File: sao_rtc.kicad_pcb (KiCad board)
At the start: 2 copper layers, 44.9 x 32.9 mm, 40 parts, among them J1 S2B-PH-K-S(LF)(SN), J2 Conn_02x03_Odd_Even, J3 Conn_02x03_Odd_Even, P1 USB_C_Plug_USB2.0, SW1 DPDT, U1 AW32001ECSR, U2 PCF8563DRG, U3 M3410, Y1 32.768 kHz

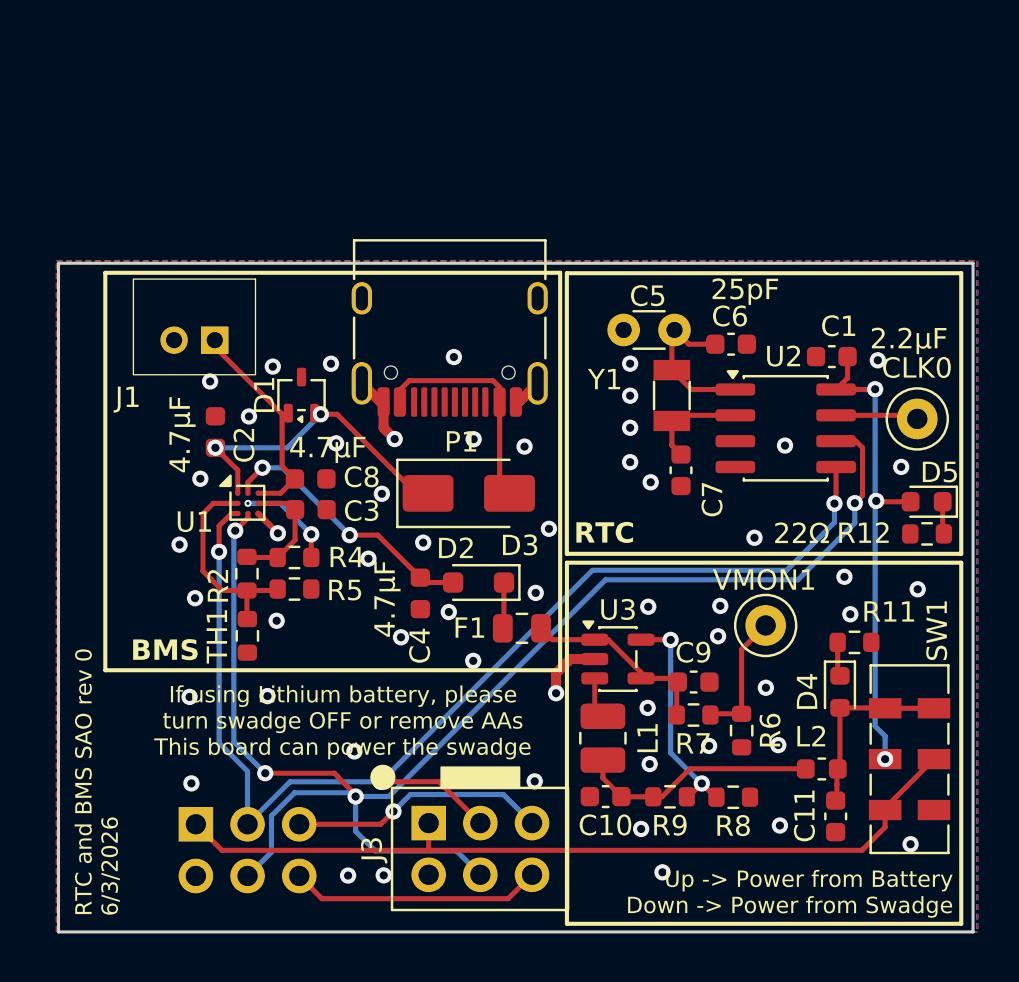
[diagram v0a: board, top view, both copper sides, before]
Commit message: Complete 1st Draft
First Draft at Schematic Capture and Layout
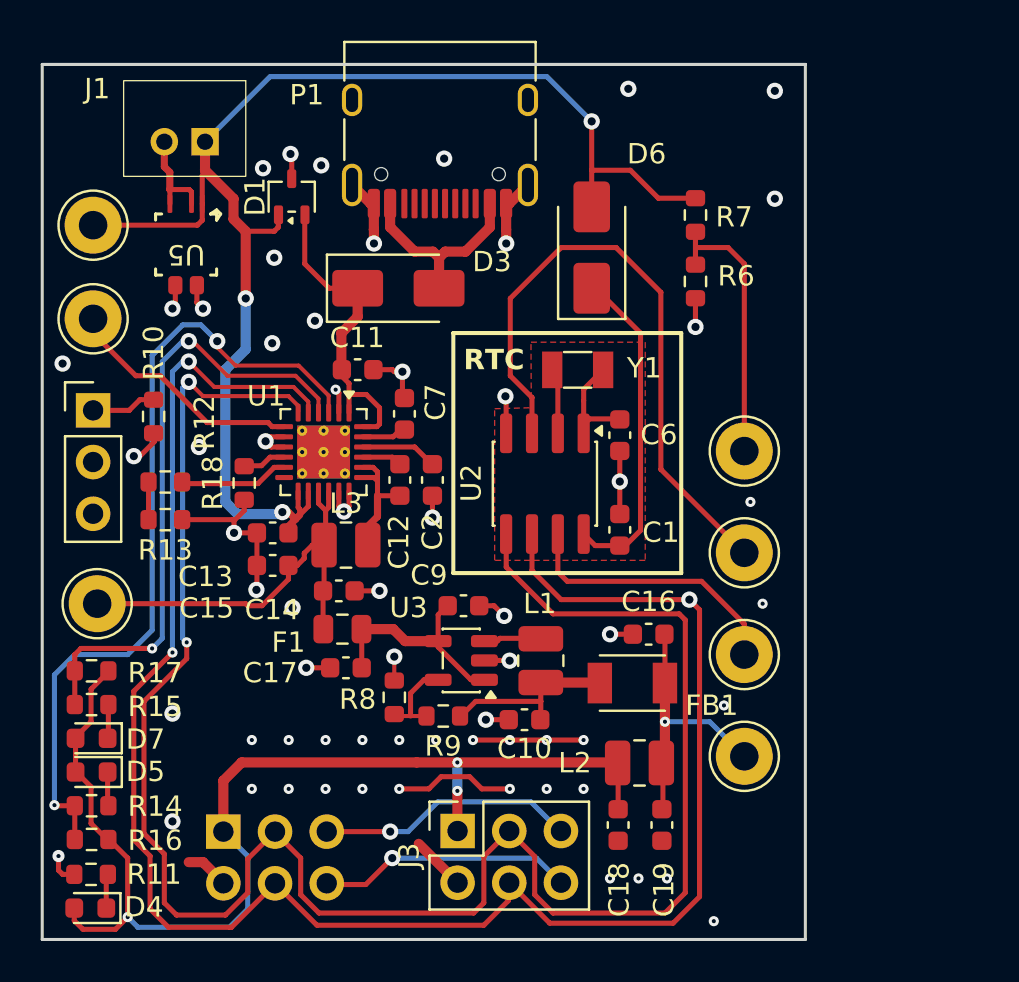
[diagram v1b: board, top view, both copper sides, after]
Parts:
- removed C3: 1μF, sao:C_0603_1608Metric
- removed C4, C8: 4.7μF, sao:C_0603_1608Metric
- removed C5: C, Capacitor_THT:C_Disc_D3.0mm_W1.6mm_P2.50mm
- removed CLK0, VMON1: TestPoint, TestPoint:TestPoint_Loop_D2.50mm_Drill1.0mm
- removed D2: 4.3V, Diode_SMD:D_SOD-323_HandSoldering
- removed R2, R5: Ω, Resistor_SMD:R_0603_1608Metric
- removed R4: 10kΩ, Resistor_SMD:R_0603_1608Metric
- removed SW1: DPDT, Button_Switch_SMD:SW_DPDT_CK_JS202011JCQN
- removed TH1: Thermistor_NTC, Resistor_SMD:R_0603_1608Metric
- added C12: 47nF, Capacitor_SMD:C_0603_1608Metric, F.Cu at (97.6, 71.4)
- added C13: 10uF, Capacitor_SMD:C_0603_1608Metric, F.Cu at (91.3, 74.0)
- added C14: 10uF, Capacitor_SMD:C_0603_1608Metric, F.Cu at (94.6, 76.9)
- added C15: 10uF, Capacitor_SMD:C_0603_1608Metric, F.Cu at (91.3, 75.6)
- added C16: 22uF, Capacitor_SMD:C_0603_1608Metric, F.Cu at (109.8, 79.0)
- added C17: 22uF, Capacitor_SMD:C_0603_1608Metric, F.Cu at (94.9, 80.7)
- added C18: 47nF, Capacitor_SMD:C_0603_1608Metric, F.Cu at (108.3, 88.4)
- added C19: 47nF, Capacitor_SMD:C_0603_1608Metric, F.Cu at (110.5, 88.4)
- added D6: D, Diode_SMD:D_SMA, F.Cu at (107.0, 60.0)
- added D7: STAT, LED_SMD:LED_0603_1608Metric, F.Cu at (82.4, 84.1)
- added FB1: FerriteBead, Inductor_SMD:L_TDK_NLV32_3.2x2.5mm, F.Cu at (109.0, 81.4)
- added JP1: PH2.54-1x3P, Connector_PinHeader_2.54mm:PinHeader_1x03_P2.54mm_Vertical, F.Cu at (82.5, 68.0)
- added L3: 1uH, Inductor_SMD:L_1008_2520Metric, F.Cu at (94.9, 74.6)
- added R10: 10kΩ, Resistor_SMD:R_0603_1608Metric, F.Cu at (85.5, 68.3)
- added R12: 5.36k, Resistor_SMD:R_0603_1608Metric, F.Cu at (86.0, 71.5)
- added R13: 31.6k, Resistor_SMD:R_0603_1608Metric, F.Cu at (86.0, 73.4)
- added R15: 22Ω, Resistor_SMD:R_0603_1608Metric, F.Cu at (82.4, 82.5)
- added R16: 10kΩ, Resistor_SMD:R_0603_1608Metric, F.Cu at (82.4, 89.1)
- added R17: 10kΩ, Resistor_SMD:R_0603_1608Metric, F.Cu at (82.4, 80.8)
- added R18: 232, Resistor_SMD:R_0603_1608Metric, F.Cu at (89.9, 71.6)
- added TP1: TestPoint, TestPoint:TestPoint_Loop_D2.60mm_Drill1.4mm_Beaded, F.Cu at (114.5, 80.0)
- added TP2: TestPoint, TestPoint:TestPoint_Loop_D2.60mm_Drill1.4mm_Beaded, F.Cu at (114.5, 75.0)
- added TP3: TP_BATT, TestPoint:TestPoint_Loop_D2.60mm_Drill1.4mm_Beaded, F.Cu at (82.5, 58.9)
- added TP4: TP_PGOOD, TestPoint:TestPoint_Loop_D2.60mm_Drill1.4mm_Beaded, F.Cu at (82.5, 63.5)
- added TP5: TP_BMS, TestPoint:TestPoint_Loop_D2.60mm_Drill1.4mm_Beaded, F.Cu at (82.7, 77.5)
- added TP6: TP_VMON, TestPoint:TestPoint_Loop_D2.60mm_Drill1.4mm_Beaded, F.Cu at (114.5, 70.0)
- added TP7: TP_3V3, TestPoint:TestPoint_Loop_D2.60mm_Drill1.4mm_Beaded, F.Cu at (114.5, 85.0)
- added U5: XB7608AJ, sao:CPC-5_2.6mmx4mm_P0.53mm, F.Cu at (87.1, 59.9)
- C1: value 2.2μF -> 22uF
- C11: value 12uF -> 1μF
- C2: footprint sao:C_0603_1608Metric -> Capacitor_SMD:C_0603_1608Metric
- C7: value ~ -> 10μF
- D5: value RTC ON -> PGOOD
- J2: value Conn_02x03_Odd_Even -> Connector, In
- J3: value Conn_02x03_Odd_Even -> Connector, Out; footprint Swadge_Parts:PinSocket_2x03_P2.54mm_Vertical -> sao:PinHeader_2x03_P2.54mm_Vertical_Flipped
- L2: footprint Inductor_SMD:L_0603_1608Metric -> Inductor_SMD:L_1008_2520Metric
- U1: value AW32001ECSR -> BQ24259; footprint Package_CSP:WLCSP-9_1.21x1.22mm_Layout3x3_P0.4mm -> Package_DFN_QFN:HVQFN-24-1EP_4x4mm_P0.5mm_EP2.6x2.6mm_ThermalVias
- U3: value M3410 -> MT3410
- moved R14 43.2 mm to (82.4, 87.4)
- moved D5 43.1 mm to (82.4, 85.8)
- moved R11 39.2 mm to (82.4, 90.8), turned to 0 degrees
- moved D4 38.3 mm to (82.4, 92.5), turned to 180 degrees
- moved C11 32.1 mm to (95.5, 66.0), turned to 0 degrees
- moved R7 24.6 mm to (112.1, 58.4), turned to 90 degrees
- moved R6 22.2 mm to (112.1, 61.7)
- moved R8 17.4 mm to (97.3, 82.1), turned to -90 degrees
- moved C7 13.9 mm to (97.8, 68.2), turned to 90 degrees
- moved C1 13.5 mm to (108.4, 73.9), turned to 90 degrees
- moved U2 12.1 mm to (104.7, 71.6), turned to -90 degrees
- moved C9 11.9 mm to (100.7, 77.6)
- moved R9 11.8 mm to (99.7, 83.0), turned to 0 degrees
- moved C2 10.9 mm to (99.2, 71.4), turned to -90 degrees
- moved D3 10.7 mm to (97.5, 62.0)
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- renumbered R12 to R14
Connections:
- net Net-(U2-OSCI) renamed /RTC/OSCI
- net Net-(U3-FB) renamed /3V3_REG/FB
- C1 pad 1: VDD -> /RTC/V_RTC
- C10 pad 1: Net-(C10-Pad1) -> /3V3_REG/3V3_SW
- C11 pad 1: 3V3 SAO -> +5V
- C2 pad 1: +5V -> /BMS/REGN
- C7 pad 1: Net-(U2-OSCO) -> /BMS/PMID
- C9 pad 1: SNODE -> /VBMS
- D1 pad 1: BATT+ -> /BATT+
- D4 pad 2: 3V3 SAO -> 3V3
- D5 pad 2: VDD -> 3V3
- F1 pad 1: SNODE -> /BMS/VSYS
- F1 pad 2: Net-(D2-K) -> /VBMS
- J1 pad 1: BATT+ -> /BATT+
- J1 pad 2: GND -> Net-(J1-Pad2)
- J2 pad 3: SDA -> /SDA
- J2 pad 4: SCL -> /SCL
- J3 pad 3: SDA -> /SDA
- J3 pad 4: SCL -> /SCL
- L1 pad 1: Net-(C10-Pad1) -> /3V3_REG/3V3_SW
- L2 pad 1: 3V3 SAO -> 3V3
- L2 pad 2: Net-(C10-Pad1) -> /3V3_SAO
- R14 pad 1: GND -> /~{PG}
- R7 pad 2: SNODE -> /BATT+
- R9 pad 2: Net-(C10-Pad1) -> /3V3_REG/3V3_SW
- U2 pad 2: Net-(U2-OSCO) -> /RTC/OSCO
- U2 pad 3: unconnected-(U2-~{INT}-Pad3) -> /RTC/~{INT}
- U2 pad 5: SDA -> /SDA
- U2 pad 6: SCL -> /SCL
- U2 pad 7: Net-(U2-CLKO) -> /RTC/CLK0
- U2 pad 8: VDD -> /RTC/V_RTC
- U3 pad 1: SNODE -> /VBMS
- U3 pad 4: SNODE -> /VBMS
- Y1 pad 1: Net-(U2-OSCO) -> /RTC/OSCO
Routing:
- net /SDA: track 0.00 -> 95.7 mm, vias 0 -> 2
- net /SCL: track 0.00 -> 92.6 mm, vias 0 -> 3
- net SCL: track 71.0 -> 0.00 mm, vias 4 -> 0
- net /BATT+: track 0.00 -> 69.2 mm, vias 0 -> 3
- net SDA: track 59.9 -> 0.00 mm, vias 3 -> 0
- net GND: track 9.49 -> 62.5 mm, vias 54 -> 63
- net /~{PG}: track 0.00 -> 40.1 mm, vias 0 -> 2
- net /RTC/~{INT}: track 0.00 -> 30.9 mm
- net /STAT: track 0.00 -> 30.6 mm, vias 0 -> 2
- net VDD: track 23.9 -> 0.00 mm, vias 3 -> 0
- net /BMS/VSYS: track 0.00 -> 21.0 mm
- net /RTC/V_RTC: track 0.00 -> 16.3 mm
- net 3V3: track 40.6 -> 56.5 mm, vias 0 -> 3
- net /RTC/CLK0: track 0.00 -> 13.6 mm
- net Net-(D2-A): track 13.3 -> 0.00 mm, vias 2 -> 0
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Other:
- board size 44.9 x 32.9 mm -> 37.5 x 43 mm
- board text added: "If using Lithium battery, please turn swadge OFF or remove AAs This board WILL power the swadge"
- board text added: "RTC and BMS SAO rev 1 7/4/2026"
- board text removed: "BMS"
- board text removed: "If using Lithium battery, please turn swadge OFF or remove AAs This board can power the swadge"
- board text removed: "RTC and BMS SAO rev 0 6/3/2026"
- board text removed: "Up -> Power from Battery Down -> Power from Swadge"
